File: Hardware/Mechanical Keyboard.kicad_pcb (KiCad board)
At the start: 2 copper layers, 343.4 x 105.3 mm, 260 parts, among them J1 USBMINI_B05, U1 ATMEGA32U4-AU, U2 IS31FL3731-SALS2, X1 ASX4

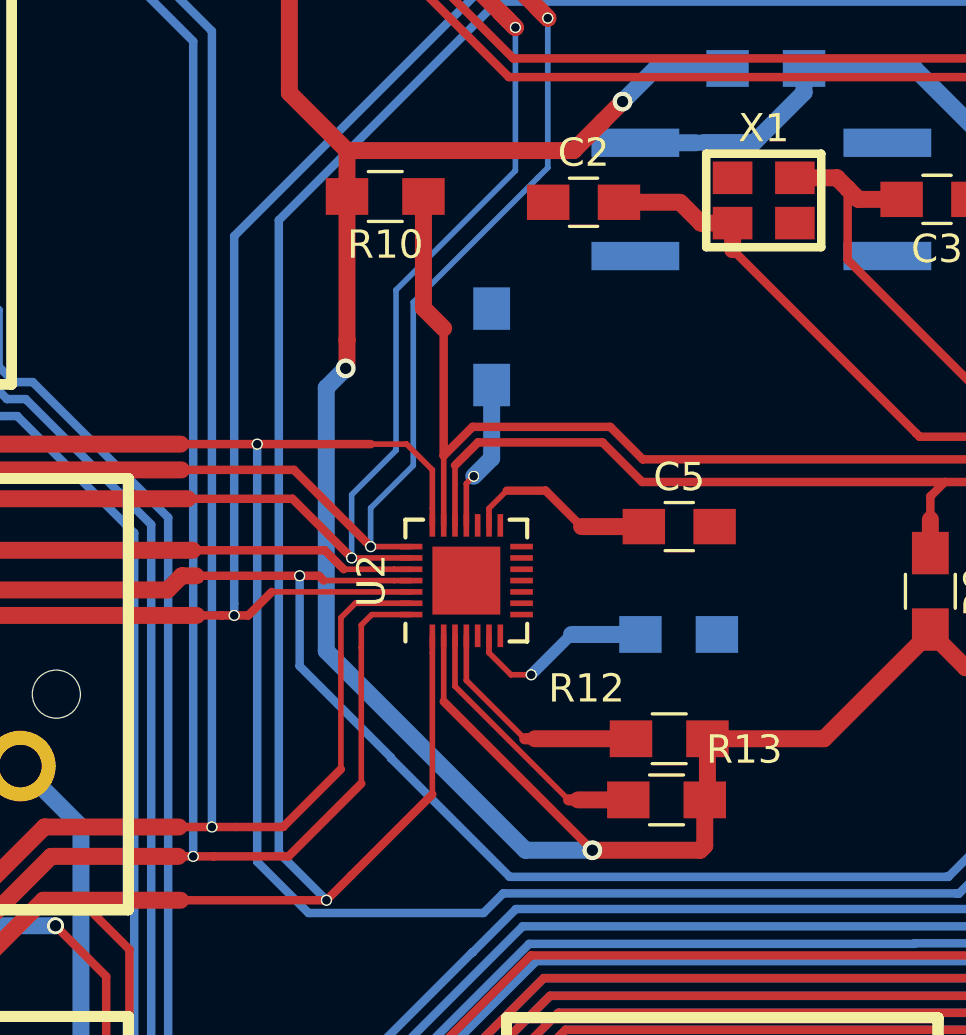
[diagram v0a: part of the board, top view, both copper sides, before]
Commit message: Small refactoring
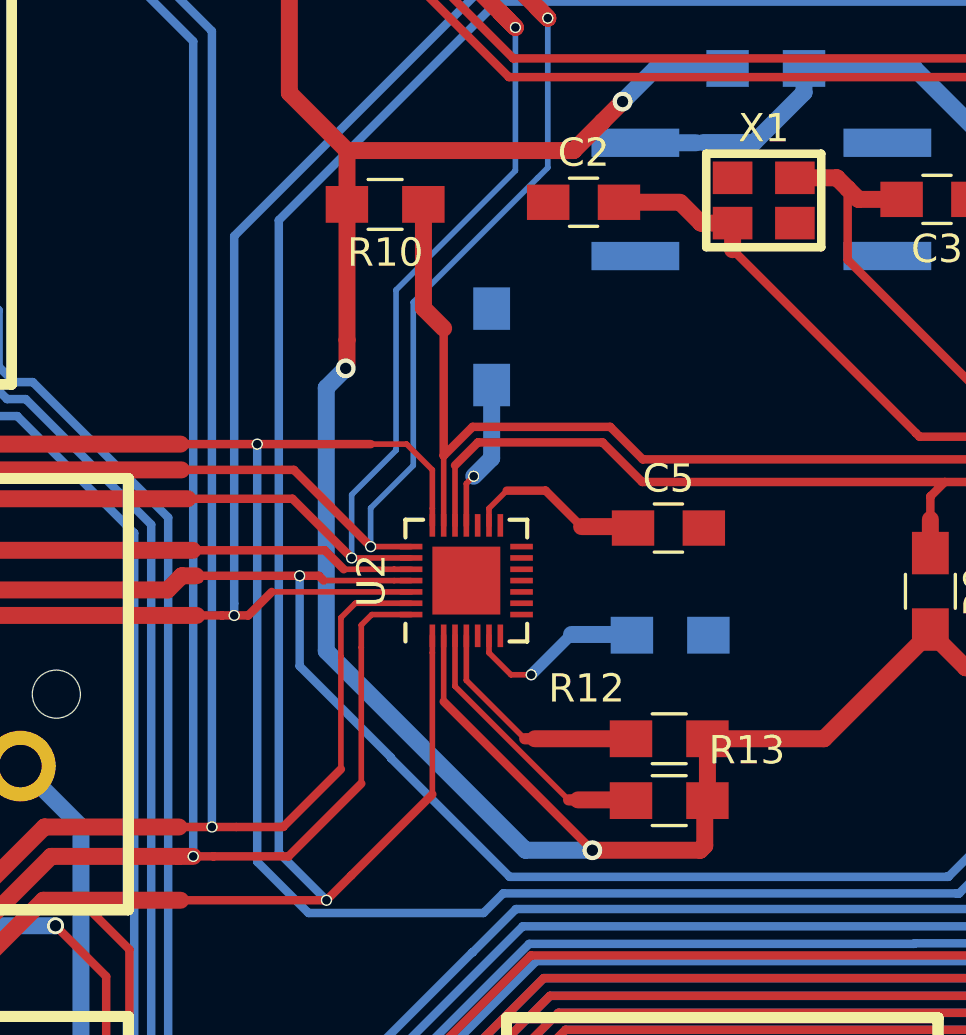
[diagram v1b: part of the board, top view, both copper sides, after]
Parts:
- moved C5 0.38 mm to (348.5, 144.7)
- moved R11 0.30 mm to (348.6, 148.5)
- moved R10 0.28 mm to (338.5, 133.3)
- moved R13 0.10 mm to (348.5, 154.3)
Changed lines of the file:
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@@
   )
   (module Capacitors_SMD:C_0805_HandSoldering (layer F.Cu)
-    (at 348.889 144.653)
+    (at 348.508 144.7038)
     (descr "Capacitor SMD 0805, hand soldering")
     (tags "capacitor 0805")
@@
   )
   (module Resistors_SMD:R_0805_HandSoldering (layer F.Cu)
-    (at 338.5058 132.9944 180)
+    (at 338.502 133.2738 180)
     (descr "Resistor SMD 0805, hand soldering")
     (tags "resistor 0805")
@@
   )
   (module Resistors_SMD:R_0805_HandSoldering (layer B.Cu)
-    (at 348.869 148.463 180)
+    (at 348.568 148.4884 180)
     (descr "Resistor SMD 0805, hand soldering")
     (tags "resistor 0805")
@@
   )
   (module Resistors_SMD:R_0805_HandSoldering (layer F.Cu)
-    (at 348.441 154.305 180)
+    (at 348.535 154.3304 180)
     (descr "Resistor SMD 0805, hand soldering")
     (tags "resistor 0805")
@@
   (segment (start 326.26 120.72) (end 326.26 122.05) (width 0.6) (layer F.Cu) (net 97))
   (via (at 326.26 122.05) (size 0.4) (drill 0.3) (layers F.Cu B.Cu) (net 97))
-  (segment (start 331.2 156.3) (end 331.724 156.3) (width 0.3) (layer F.Cu) (net 97))
   (segment (start 332.44 156.3) (end 335.09 156.3) (width 0.3) (layer F.Cu) (net 97))
   (segment (start 294.905457 80.146024) (end 360.054024 80.146024) (width 0.6) (layer F.Cu) (net 98))
@@
   (segment (start 331.724 127.514) (end 331.724 156.3) (width 0.3) (layer B.Cu) (net 97))
   (segment (start 326.26 122.05) (end 331.724 127.514) (width 0.3) (layer B.Cu) (net 97))
+  (segment (start 331.2 156.3) (end 331.724 156.3) (width 0.6) (layer F.Cu) (net 97))
   (segment (start 344.50001 103.35) (end 357.858 103.35) (width 0.6) (layer B.Cu) (net 110))
   (segment (start 357.858 103.35) (end 361.795 103.35) (width 0.6) (layer B.Cu) (net 110))
